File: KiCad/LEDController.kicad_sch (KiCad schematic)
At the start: 47 parts, among them J1 Conn_01x05, J2 UART, J3 JTAG, J5 USB_C_Receptacle_USB2.0_16P, J6 Conn_01x03, J7 VDD, J8 GND, J9 Conn_01x14, Q1 IRLZ44N, Q2 IRLZ44N, Q3 IRLZ44N, Q4 IRLZ44N, SW1 BOOT, SW2 EN, U2 ESP32-S3-WROOM-2, U3 TPS54202DDC

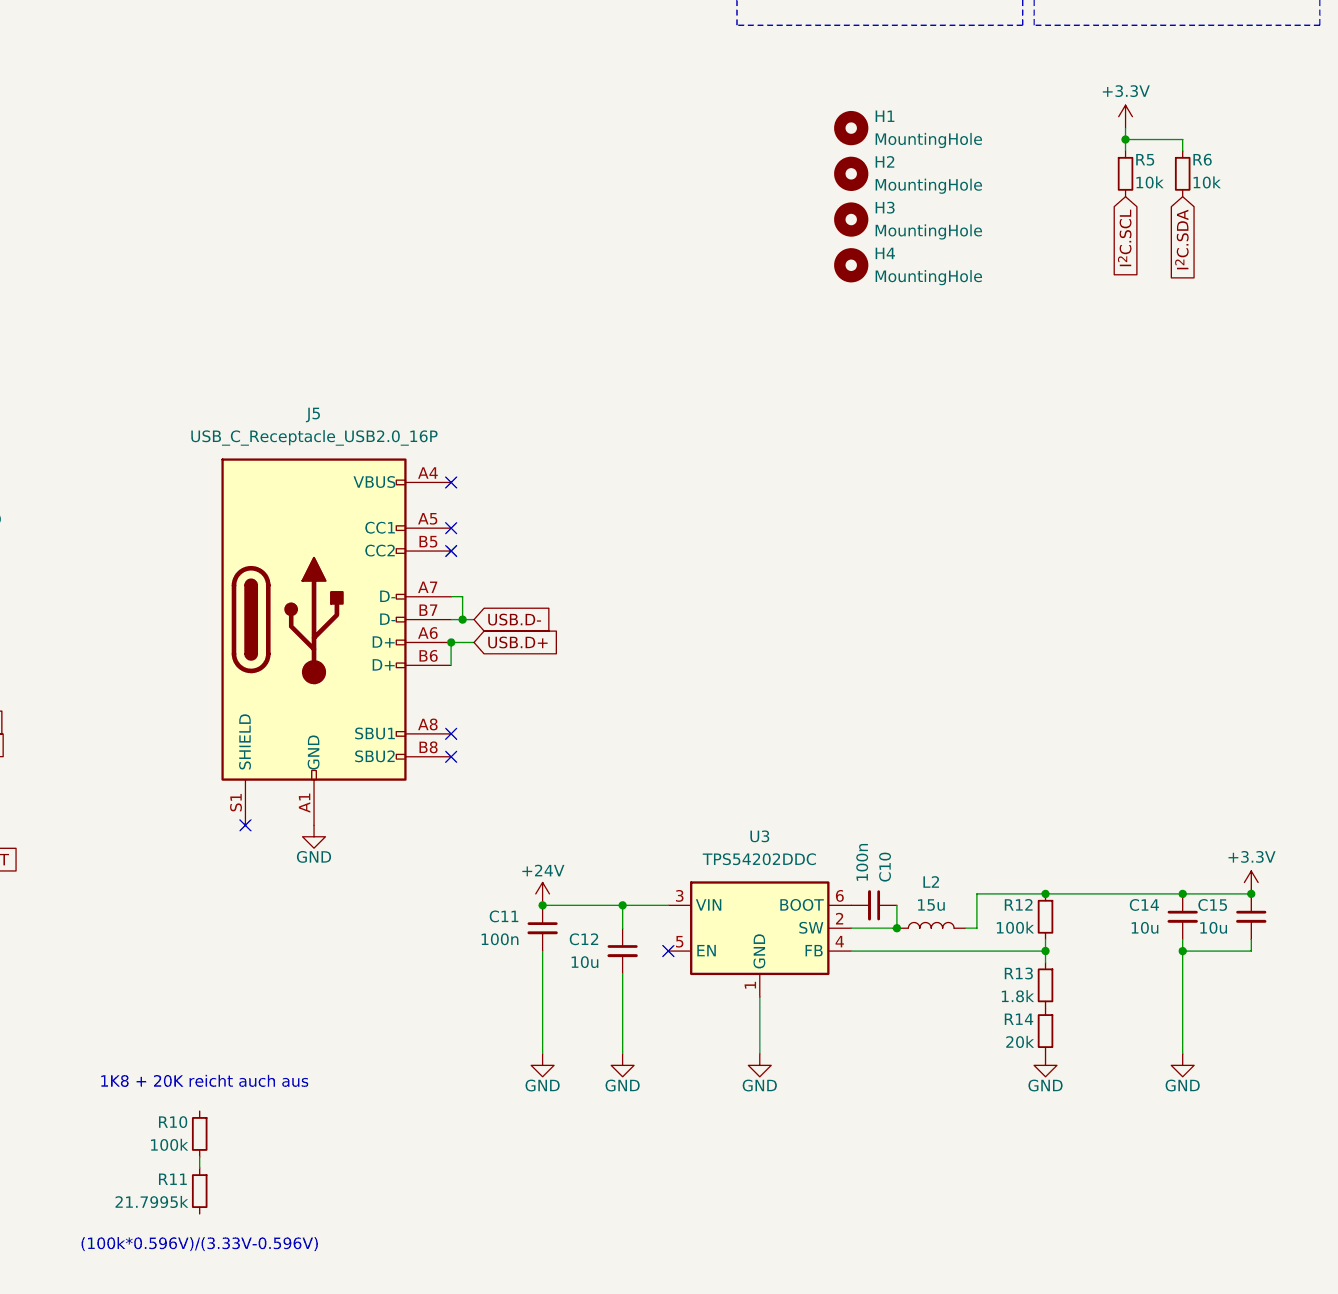
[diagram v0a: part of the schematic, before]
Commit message: .
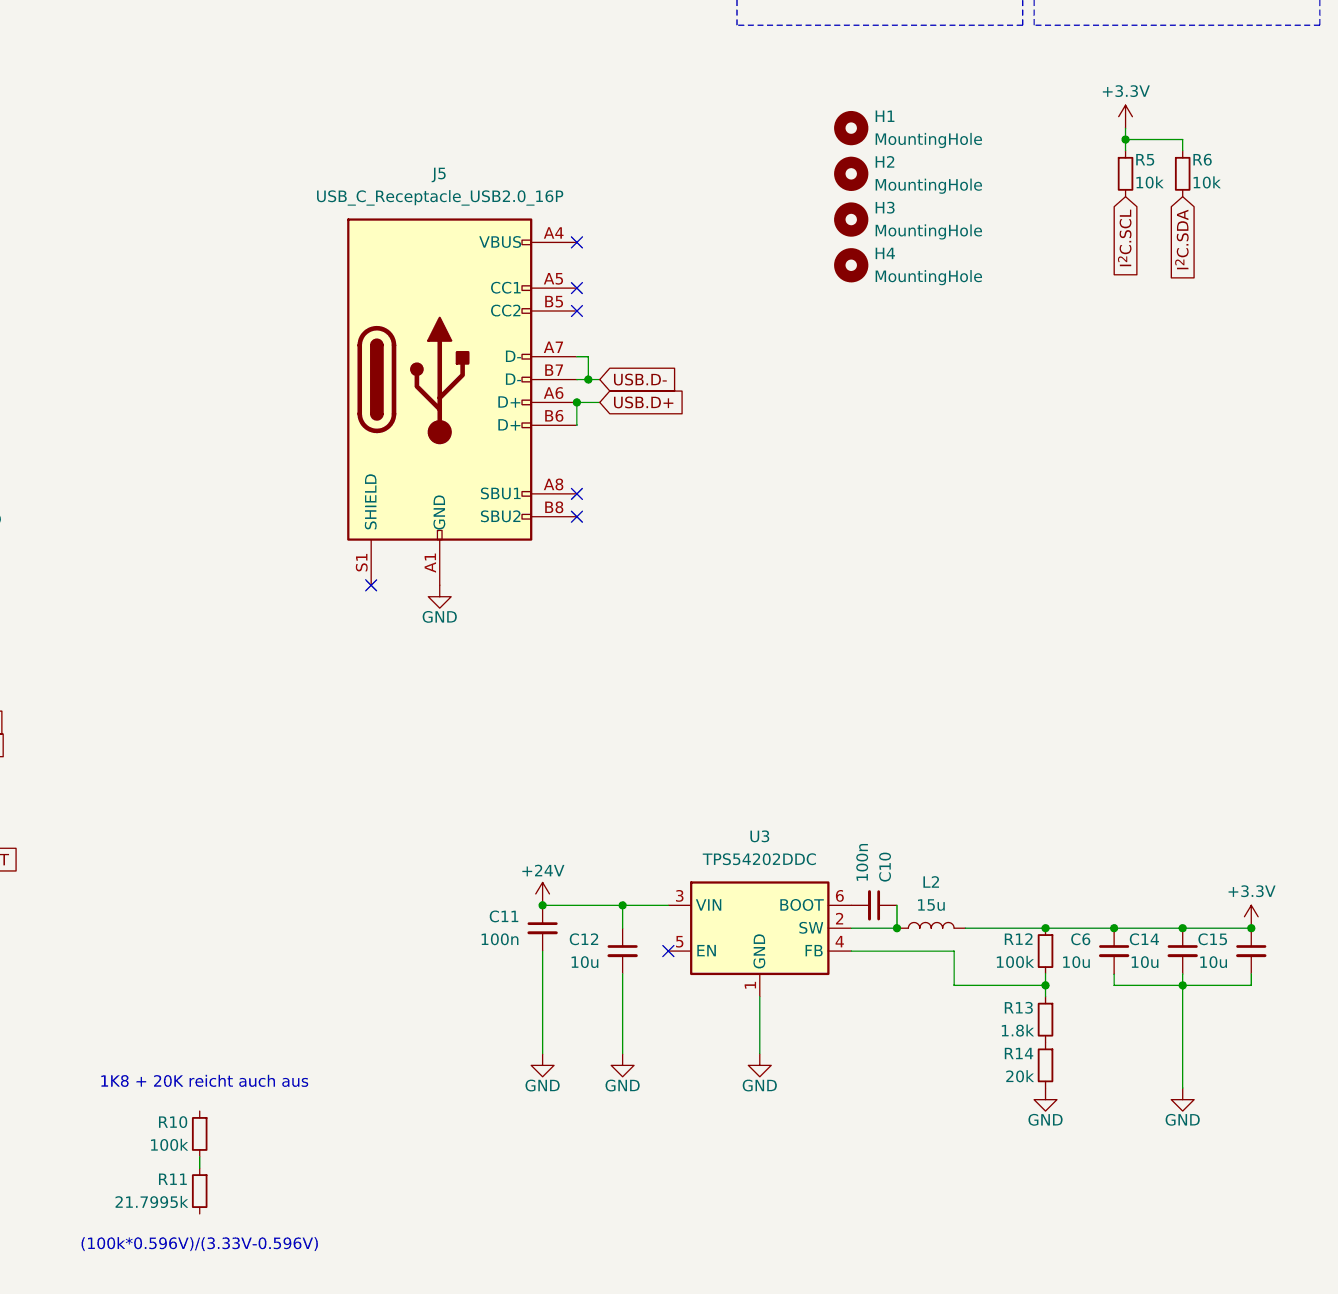
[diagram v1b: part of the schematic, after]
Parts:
- added C6: 10u, Capacitor_SMD:C_0805_2012Metric_Pad1.18x1.45mm_HandSolder, symbol Device:C_Small
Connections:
- net +3.3V: now also C6.1
- net GND: now also C6.2
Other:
- moved on the sheet: C14, C15, J5, R12, R13, R14
